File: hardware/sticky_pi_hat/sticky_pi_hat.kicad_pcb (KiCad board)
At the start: 2 copper layers, 65 x 45 mm, 41 parts, among them J1 Screw_Terminal_01x11, J2 Conn_02x13_Odd_Even, J3 Conn_01x02_Male, Q1 BSS806NH6327XTSA1, Q2 AO3415A, Q3 BSS806NH6327XTSA1, Q4 BSS806NH6327XTSA1, U2 TPL5110, U3 TPS63002, U4 DS1307Z+, U5 MCP3001-I_ST, Y1 Crystal

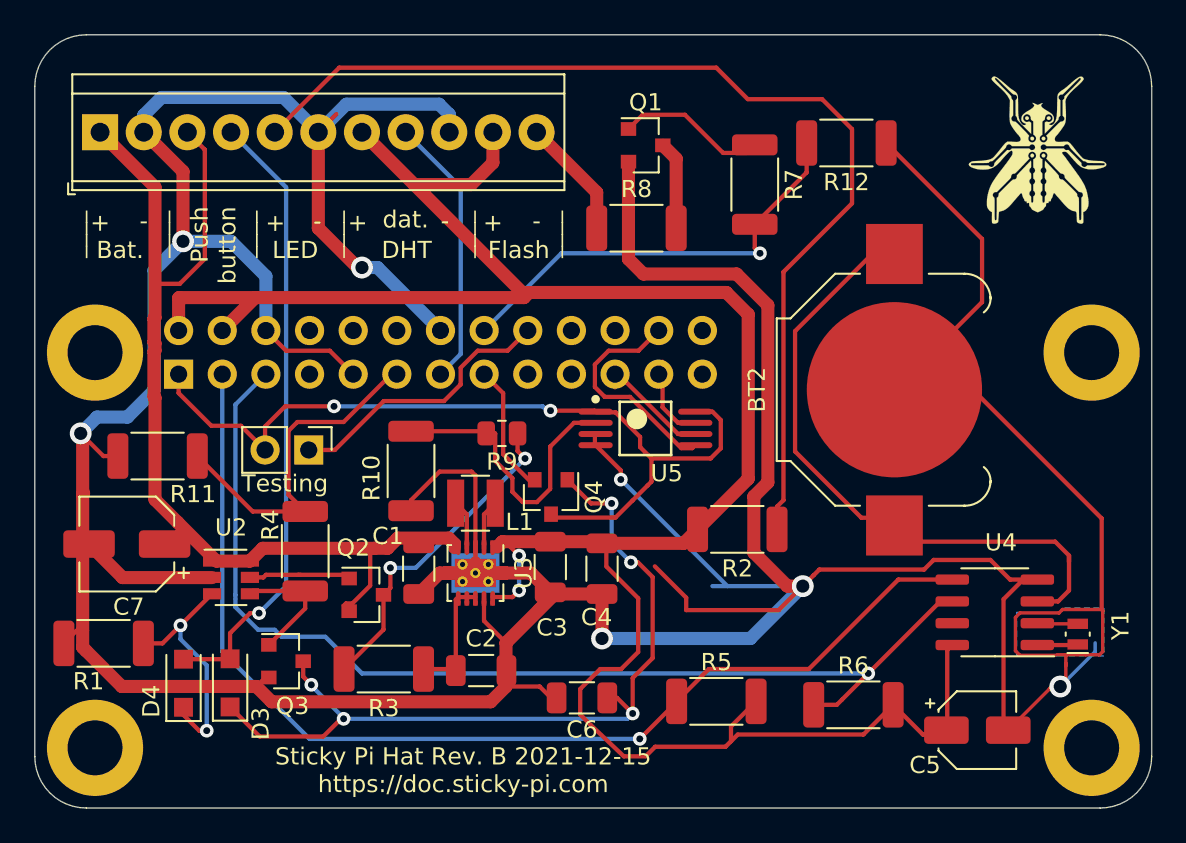
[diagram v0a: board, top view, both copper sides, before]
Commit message: hardware updates
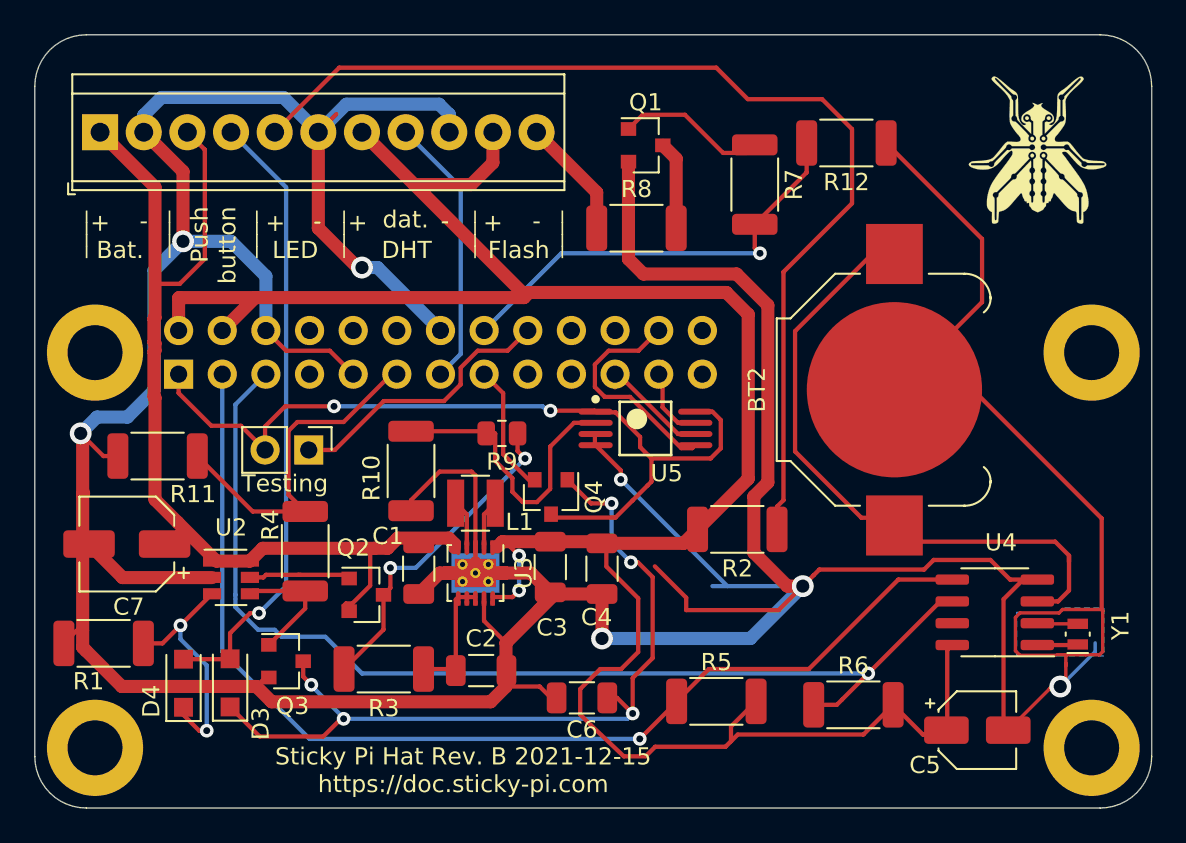
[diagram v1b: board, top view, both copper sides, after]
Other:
- net class Default removed
